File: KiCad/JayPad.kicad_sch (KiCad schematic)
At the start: 9 parts, among them SW1 SW_Push, SW2 SW_Push, SW3 SW_Push, SW4 SW_Push, SW5 SW_Push, SW6 SW_Push, U1 XIAO-RP2040-DIP

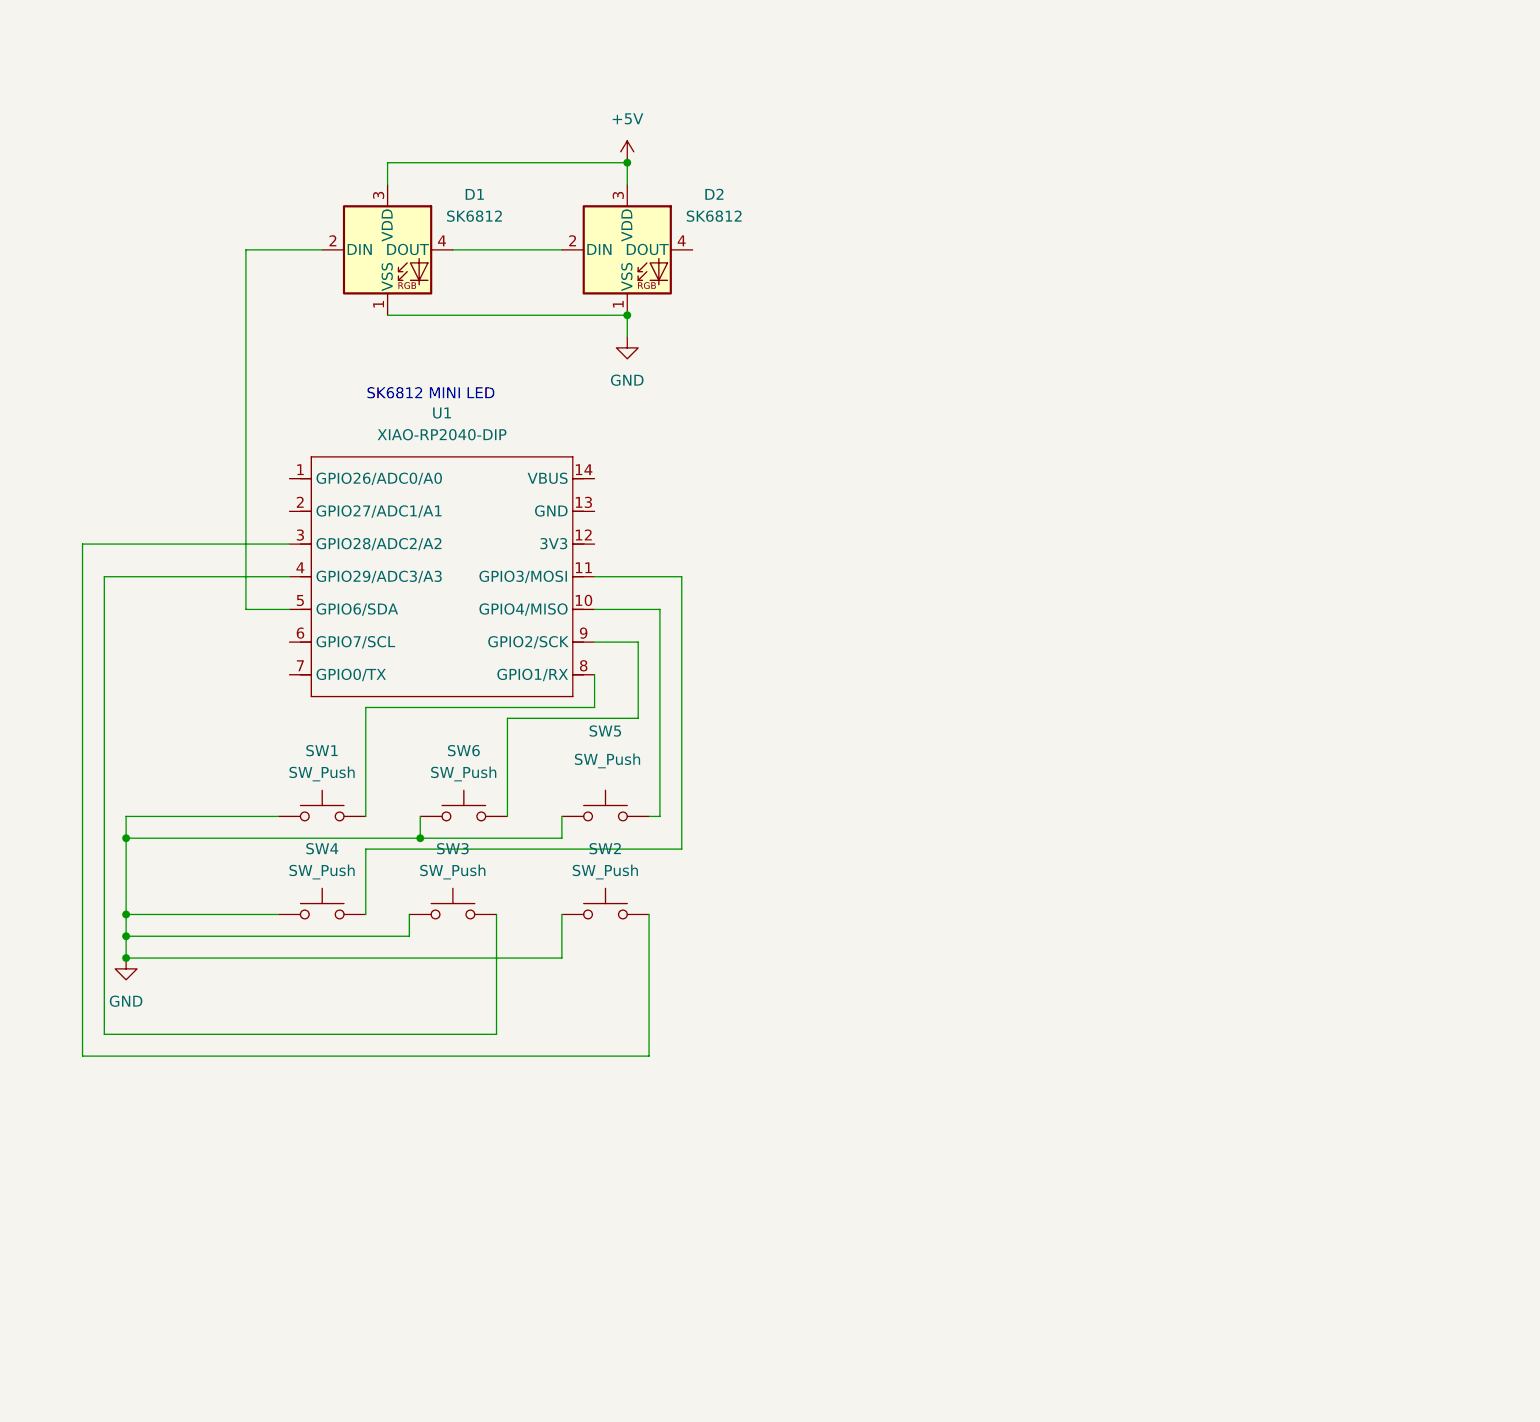
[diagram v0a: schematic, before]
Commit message: Finished Routing PCB!
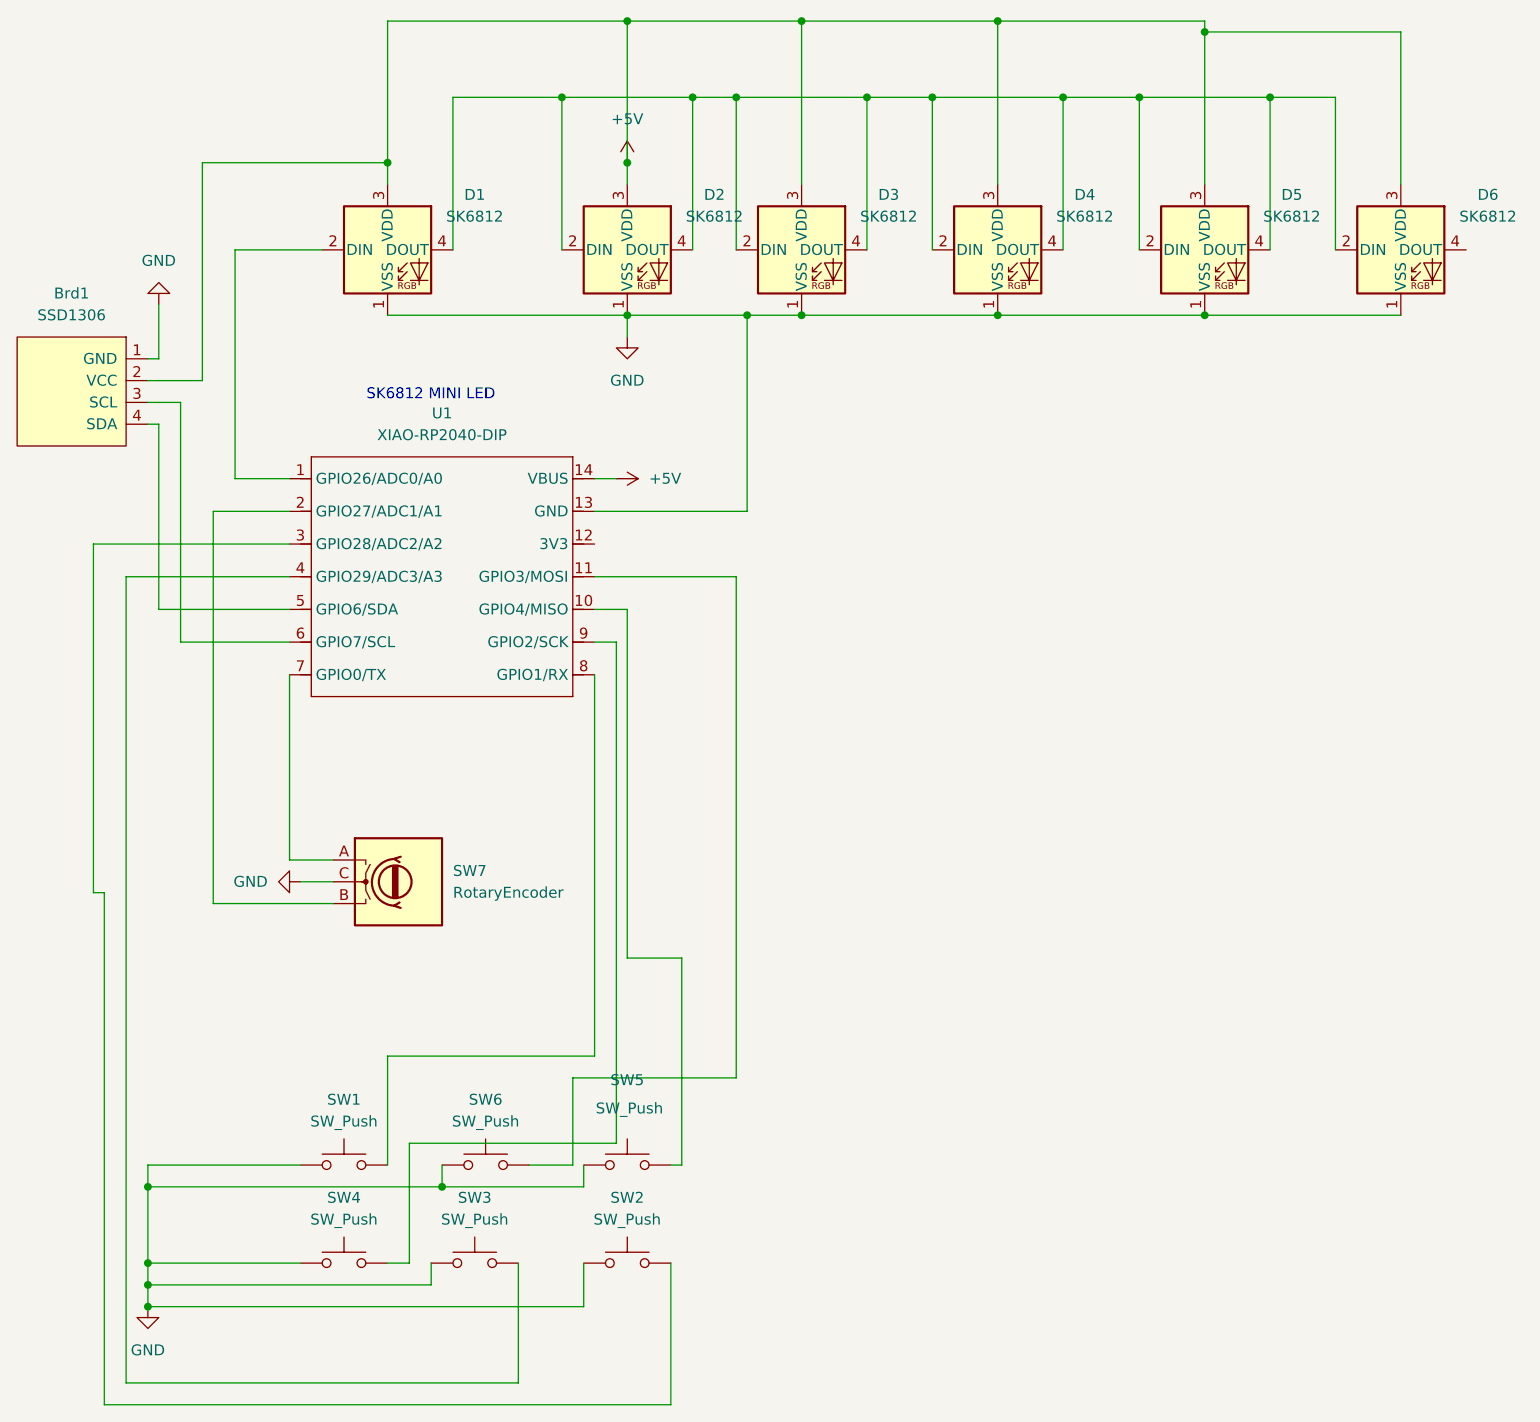
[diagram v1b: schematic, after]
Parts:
- added Brd1: SSD1306, KiCad-SSD1306-0.91-OLED-4pin-128x32.pretty-master:SSD1306-0.91-OLED-4pin-128x32, symbol SSD1306-128x64_OLED:SSD1306
- added D3, D4, D5, D6: SK6812, LED_SMD:LED_SK6812_PLCC4_5.0x5.0mm_P3.2mm, symbol LED:SK6812
- added SW7: RotaryEncoder, Rotary_Encoder:RotaryEncoder_Alps_EC11E-Switch_Vertical_H20mm, symbol Device:RotaryEncoder
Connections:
- net +5V: now also U1.14 (VBUS), Brd1.2 (VCC), D3.3 (VDD), D4.3 (VDD), D5.3 (VDD), D6.3 (VDD)
- net GND: now also U1.13 (GND), Brd1.1 (GND), D3.1 (VSS), D4.1 (VSS), D5.1 (VSS), D6.1 (VSS), SW7.C
- net at D1.2 (DIN): now also U1.1 (GPIO26/ADC0/A0); no longer U1.5 (GPIO6/SDA)
- net at D1.4 (DOUT), D2.2 (DIN): now also D2.4 (DOUT), D3.2 (DIN), D3.4 (DOUT), D4.2 (DIN), D4.4 (DOUT), D5.2 (DIN), D5.4 (DOUT), D6.2 (DIN)
- net at U1.11 (GPIO3/MOSI): now also SW6.2; no longer SW4.2
- net at U1.2 (GPIO27/ADC1/A1): now also SW7.B
- net at U1.6 (GPIO7/SCL): now also Brd1.3 (SCL)
- net at U1.7 (GPIO0/TX): now also SW7.A
- net at U1.9 (GPIO2/SCK): now also SW4.2; no longer SW6.2
- new net: Brd1.4 (SDA), U1.5 (GPIO6/SDA)
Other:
- moved on the sheet: SW1, SW2, SW3, SW4, SW5, SW6
